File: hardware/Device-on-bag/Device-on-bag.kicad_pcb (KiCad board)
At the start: 2 copper layers, 68.6 x 59.1 mm, 5 parts, among them J1 Conn_01x08, J2 Conn_01x08, J3 Conn_01x12, J4 Conn_01x12, U2 ESP32-DEVKIT-V1

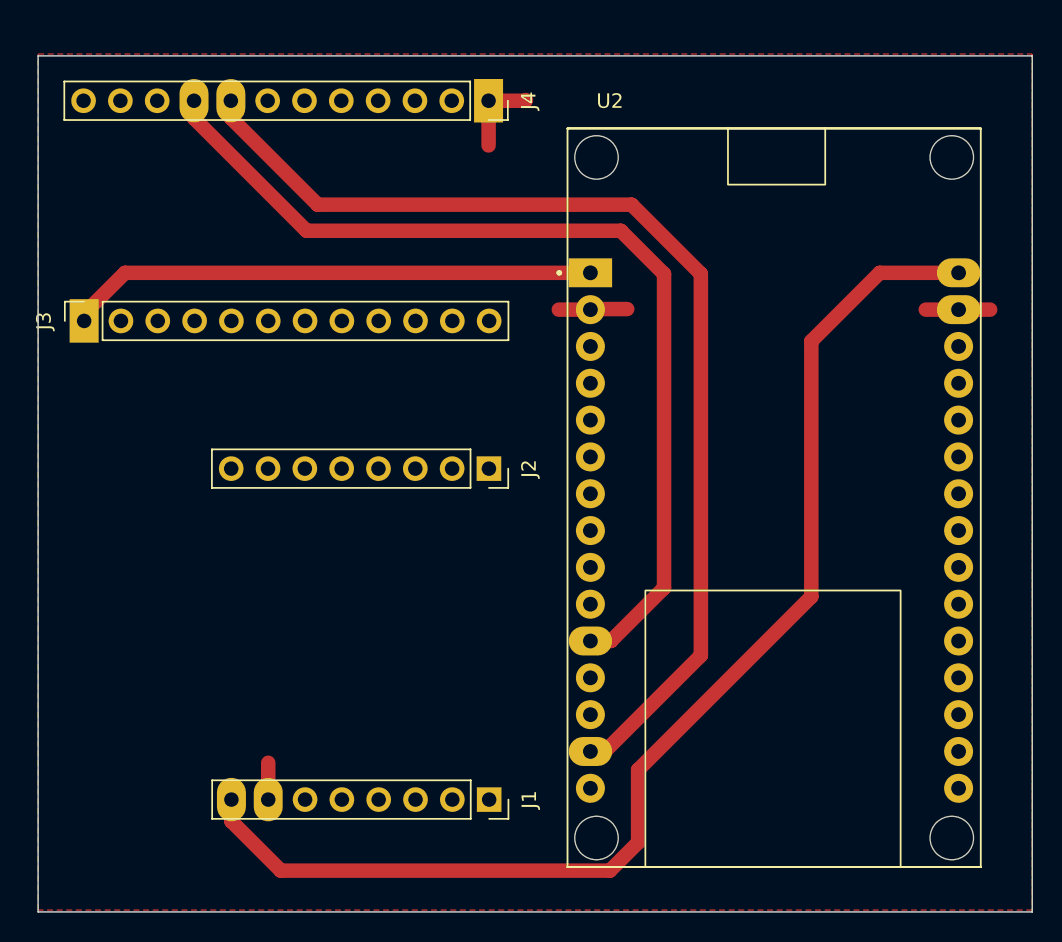
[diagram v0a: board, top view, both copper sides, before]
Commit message: update hardware
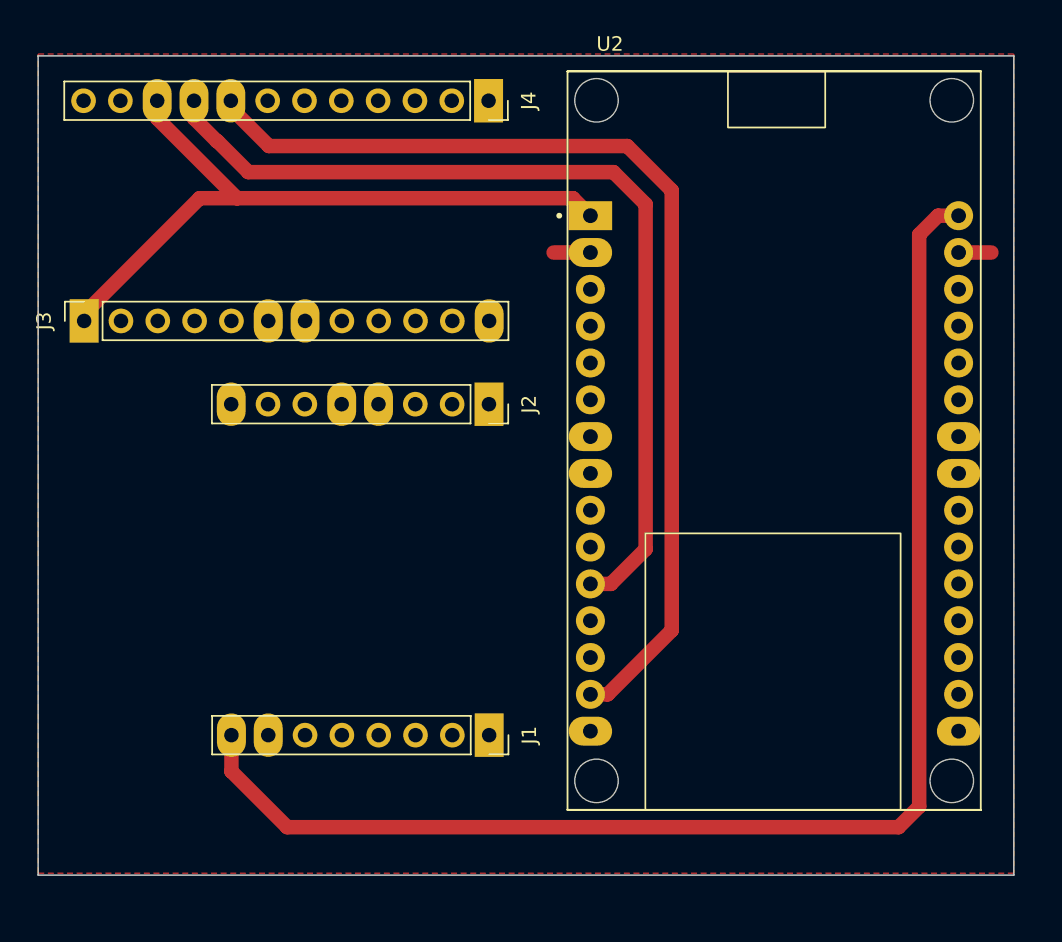
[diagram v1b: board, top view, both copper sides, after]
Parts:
- moved J1 4.45 mm to (74.3, 73.7)
- moved J2 4.45 mm to (74.3, 50.8)
- moved U2 3.94 mm to (94.0, 53.3)
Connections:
- J4 pad 10: unconnected-(J4-Pad10) -> 3.3V
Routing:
- net GND: track 17.4 -> 4.80 mm
- net 3.3V: track 36.6 -> 48.2 mm
- net Vin: track 83.4 -> 94.8 mm
- net SCL: track 75.5 -> 71.8 mm
- net SDA: track 66.3 -> 63.4 mm
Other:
- board size 68.6 x 59.1 mm -> 67.3 x 56.5 mm
